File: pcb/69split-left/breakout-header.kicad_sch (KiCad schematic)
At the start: 1 part, among them J4 Conn_01x09_Socket

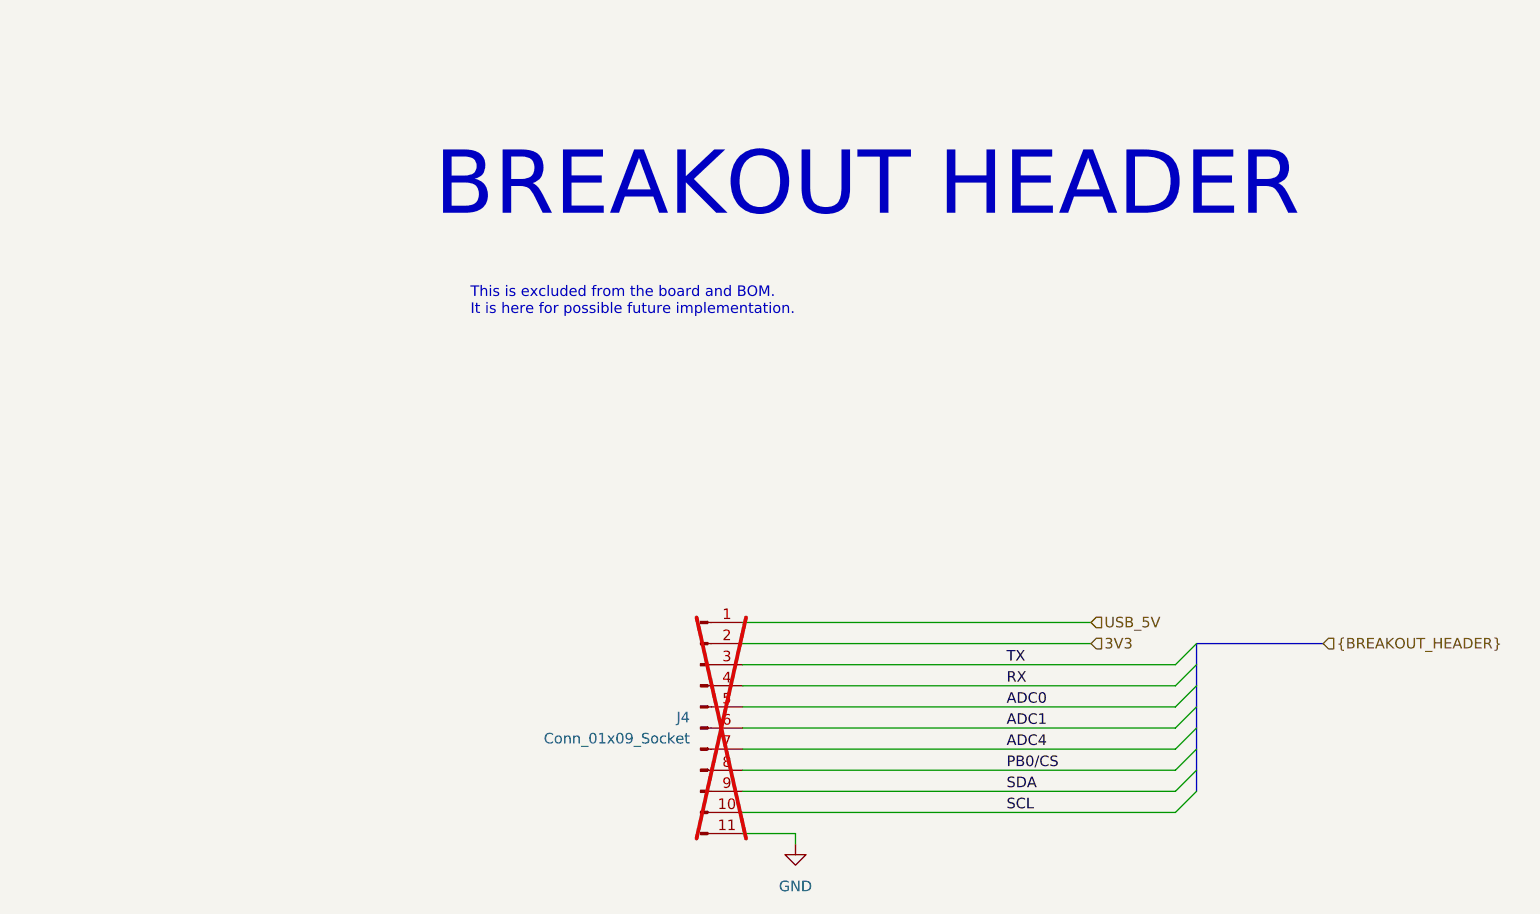
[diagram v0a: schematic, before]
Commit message: Final touches.
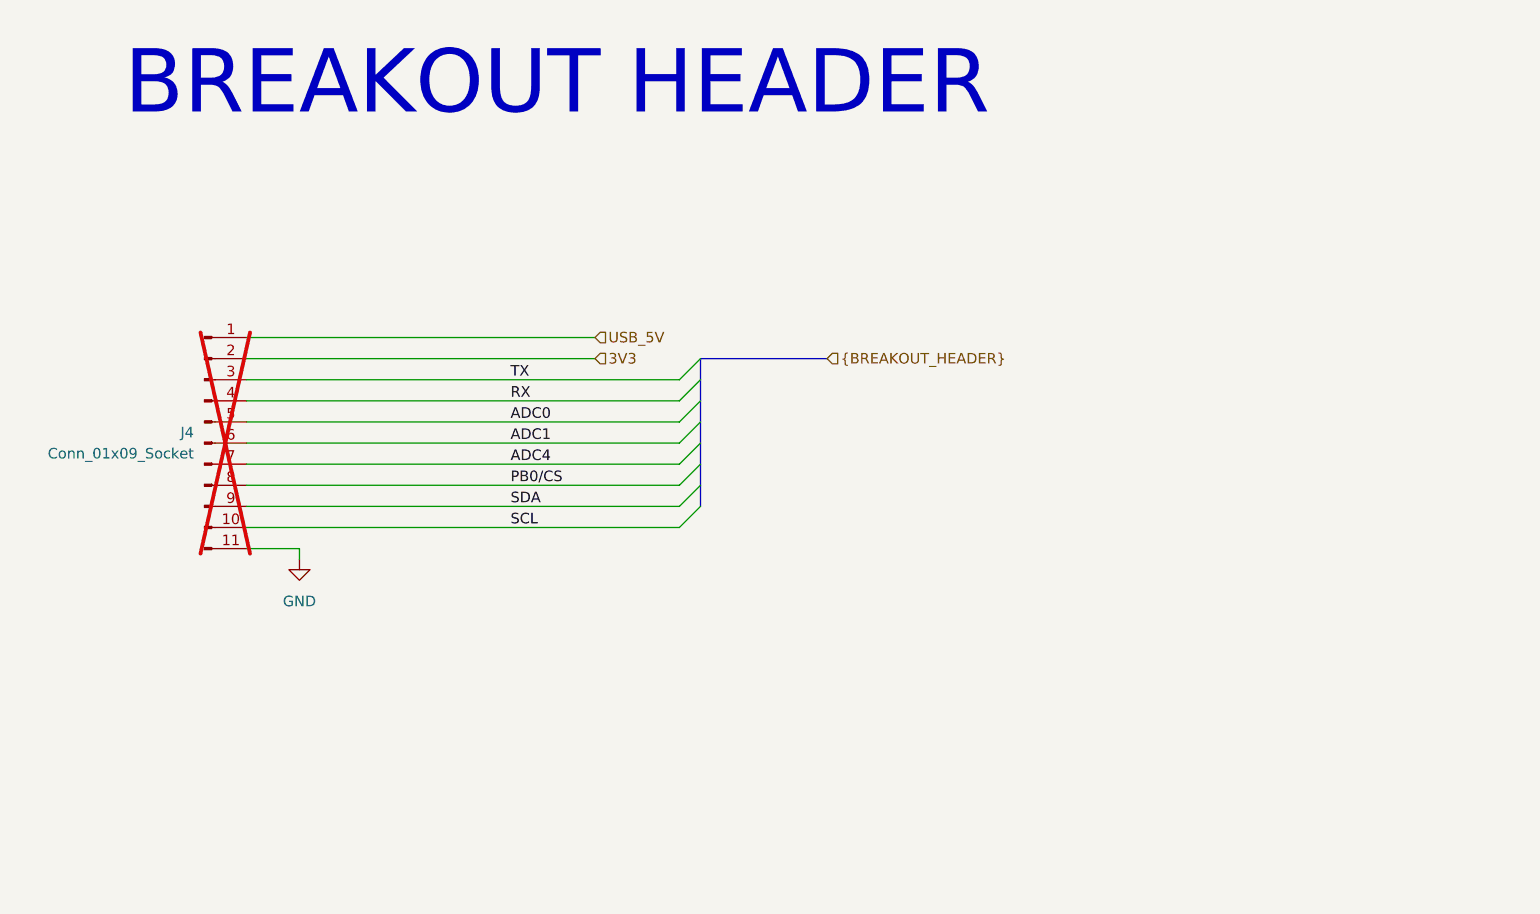
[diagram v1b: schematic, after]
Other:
- note removed: "This is excluded from the board and BOM. It is here for possible future implementation."
- moved on the sheet: J4
